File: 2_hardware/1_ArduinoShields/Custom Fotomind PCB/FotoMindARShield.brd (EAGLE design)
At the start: 160 x 100 mm, 22 parts

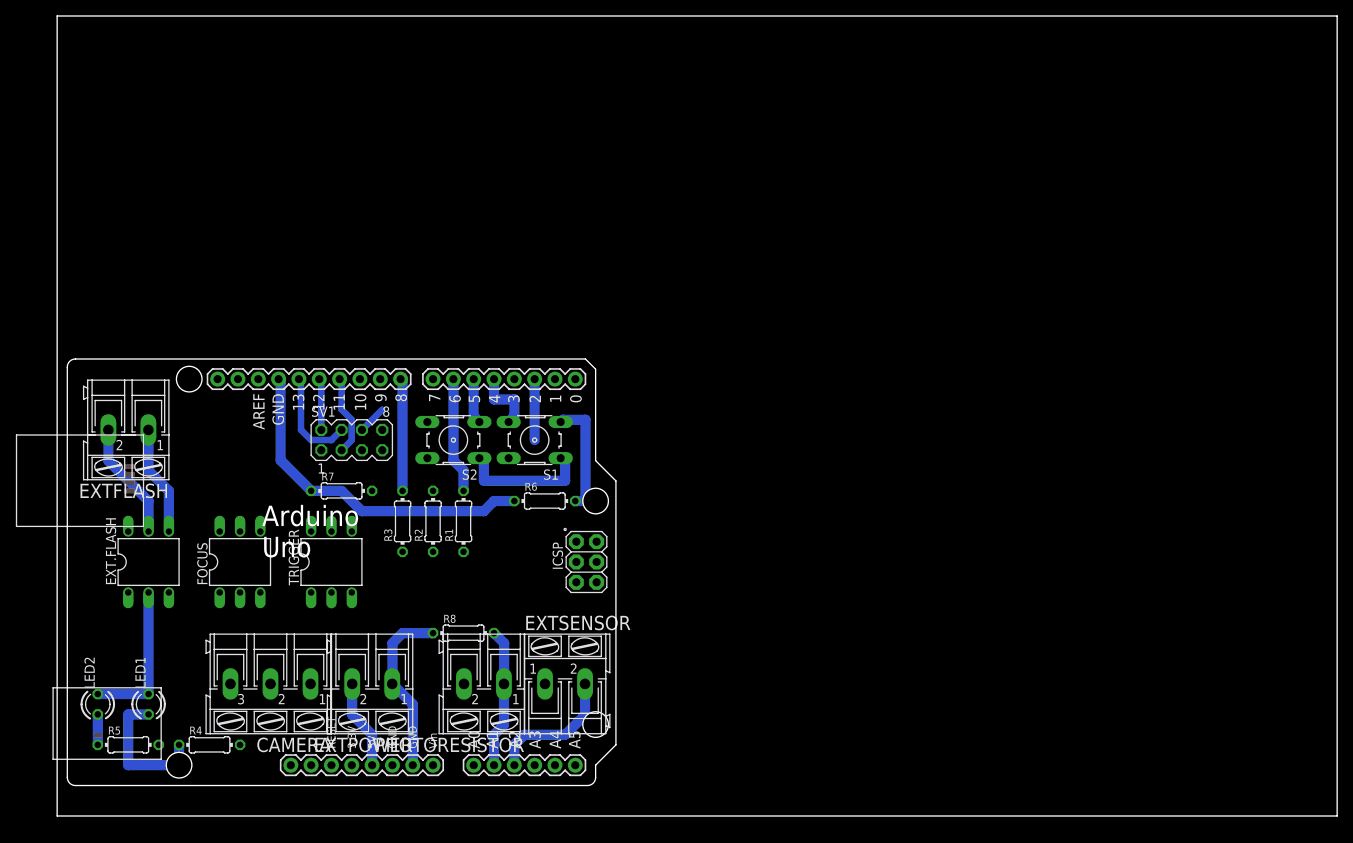
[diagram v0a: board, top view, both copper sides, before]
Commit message: Last lines PCB Shield
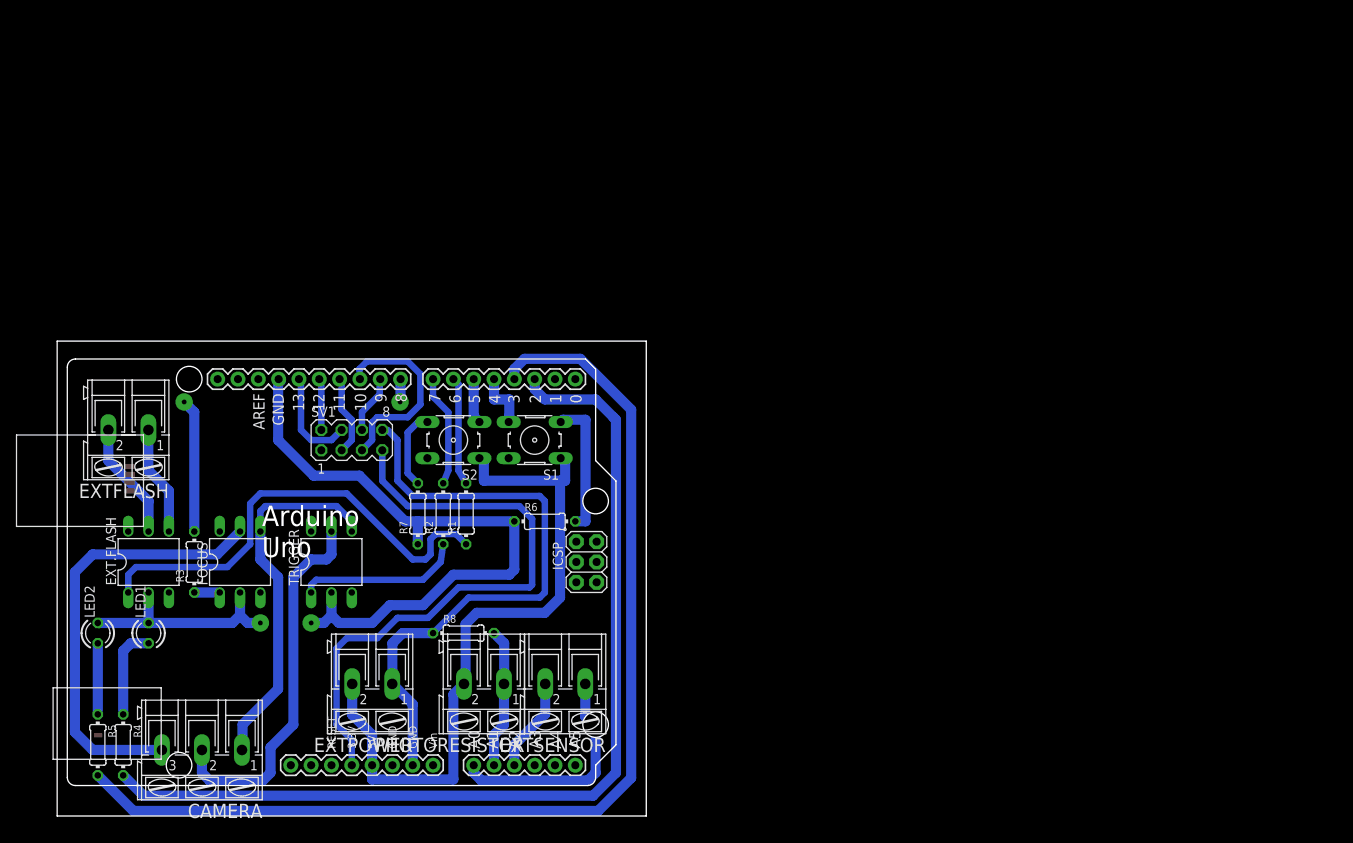
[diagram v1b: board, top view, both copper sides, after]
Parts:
- moved R3 26.5 mm to (17.1, 31.8)
- moved CAMERA 11.9 mm to (18.1, 8.26)
- moved R4 10.8 mm to (8.26, 8.89), turned to 270 degrees
- moved R7 9.94 mm to (45.1, 37.8), turned to 90 degrees
- moved LED1 8.89 mm to (11.4, 22.9)
- moved LED2 8.89 mm to (5.08, 22.9)
- moved R5 3.81 mm to (5.08, 8.89), turned to 270 degrees
- moved R6 2.54 mm to (61.0, 36.8)
- moved R2 1.59 mm to (48.3, 37.8)
- moved R1 1.00 mm to (51.1, 37.8)
- turned EXTSENSOR to 180 degrees
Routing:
- net N$8: track 0.00 -> 135.3 mm
- net N$7: track 7.62 -> 121.0 mm
- net N$30: track 0.00 -> 75.9 mm
- net N$19: track 27.6 -> 87.4 mm
- net N$1: track 0.00 -> 58.0 mm
- net N$15: track 0.00 -> 54.5 mm
- net N$21: track 21.9 -> 76.4 mm
- net GND: track 61.7 -> 110.2 mm
- net N$14: track 0.00 -> 46.7 mm
- net N$13: track 0.00 -> 46.4 mm
- net N$28: track 0.00 -> 28.6 mm
- net N$26: track 0.00 -> 24.8 mm
- net N$2: track 0.00 -> 20.6 mm
- net N$5: track 0.00 -> 13.9 mm
- net N$20: track 0.00 -> 9.88 mm
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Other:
- board size 160 x 100 mm -> 73.6 x 59.4 mm
